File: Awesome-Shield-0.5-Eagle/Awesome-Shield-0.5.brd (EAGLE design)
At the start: 100 x 80 mm, 24 parts, among them J1 ARDUINO_R3_SHIELDUNO_R3_SHIEL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, SW1 SPST_TACT-EVQQ2

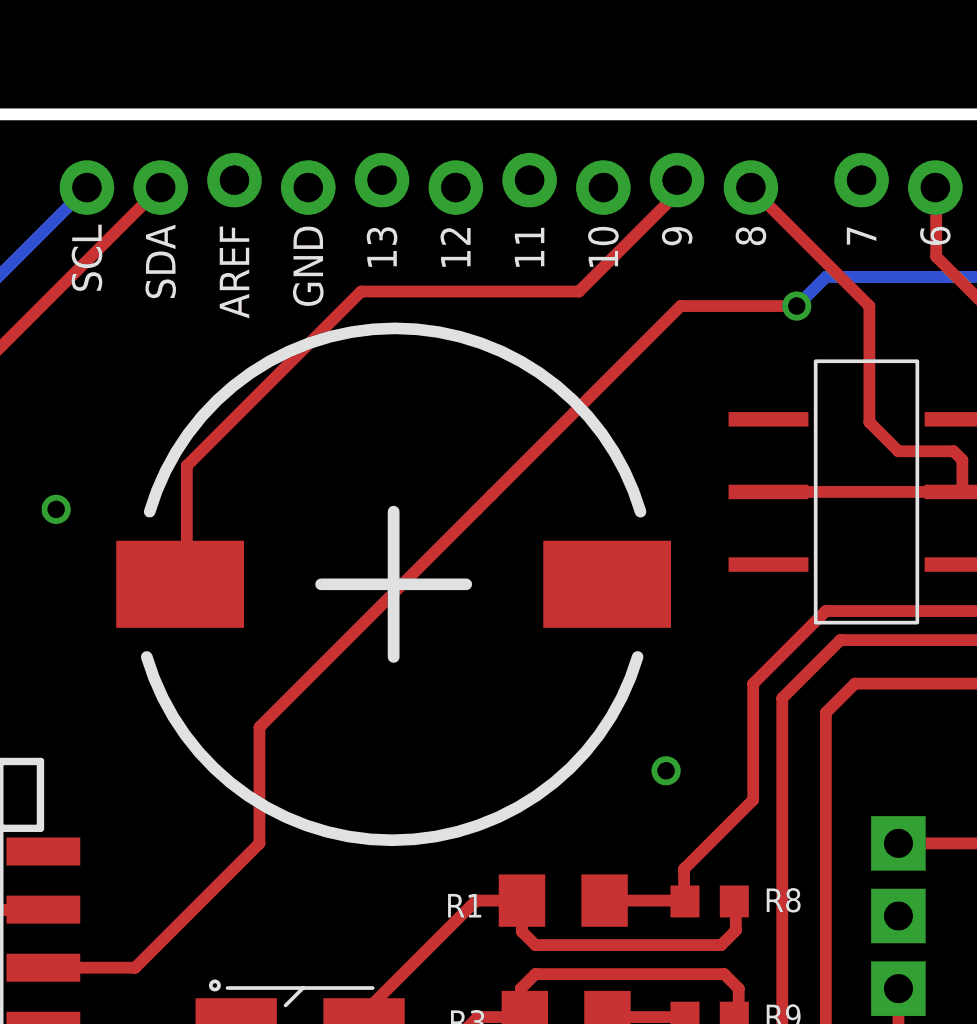
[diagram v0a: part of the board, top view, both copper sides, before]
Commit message: nudged traces
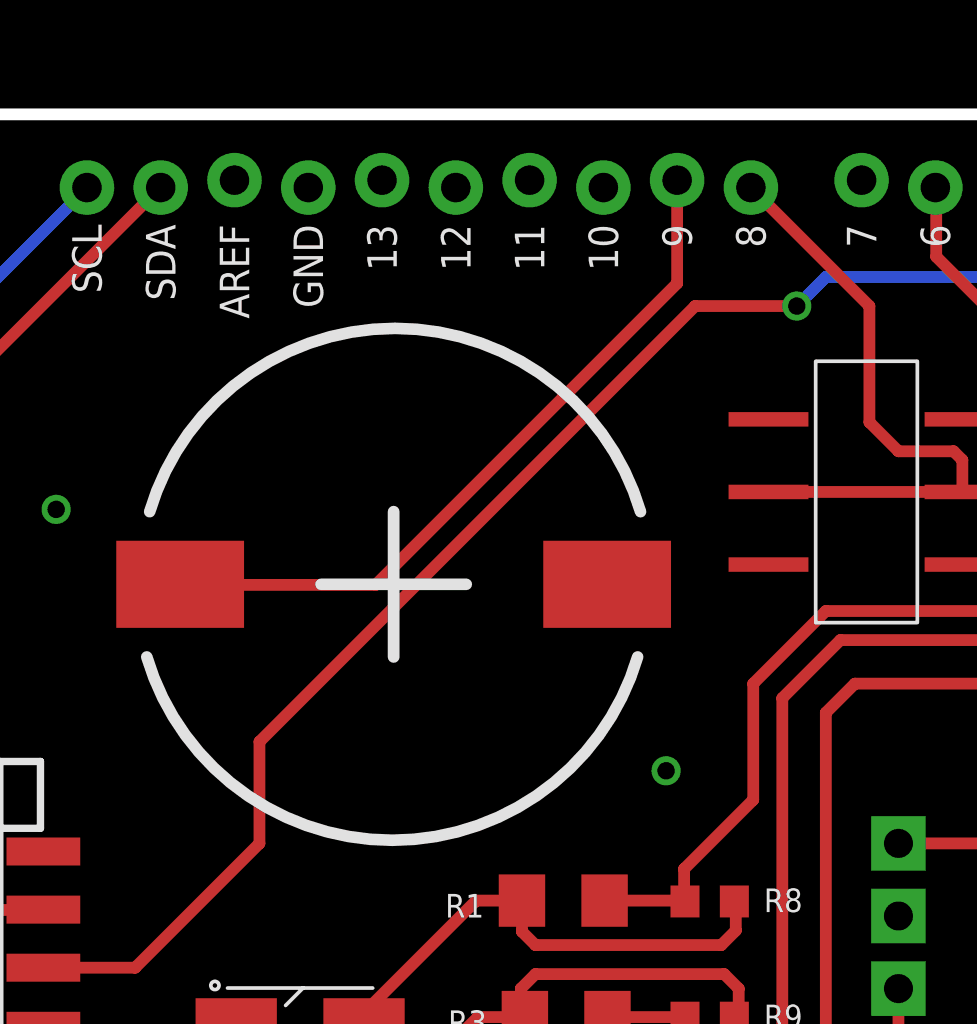
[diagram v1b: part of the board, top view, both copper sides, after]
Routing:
- net D9: track 26.9 -> 25.0 mm
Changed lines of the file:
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@@
 <via x="66.5" y="36.5" extent="1-16" drill="0.6"/>
 <via x="29.5" y="67" extent="1-16" drill="0.6"/>
+<wire x1="79.78" y1="62.58" x2="87.5" y2="73" width="0" layer="19" extent="1-1"/>
 </signal>
 <signal name="A2">
@@
 <contactref element="J1" pad="D9"/>
 <contactref element="SG1" pad="-"/>
-<wire x1="55.88" y1="68.834" x2="55.88" y2="68.38" width="0.4064" layer="1"/>
-<wire x1="55.88" y1="68.38" x2="52.5" y2="65" width="0.4064" layer="1"/>
-<wire x1="52.5" y1="65" x2="45" y2="65" width="0.4064" layer="1"/>
-<wire x1="45" y1="65" x2="39" y2="59" width="0.4064" layer="1"/>
-<wire x1="39" y1="59" x2="39" y2="54.15" width="0.4064" layer="1"/>
-<wire x1="39" y1="54.15" x2="38.77" y2="54.92" width="0.4064" layer="1"/>
+<wire x1="55.88" y1="68.834" x2="55.88" y2="65.28" width="0.4064" layer="1"/>
+<wire x1="45.5" y1="54.9" x2="38.79" y2="54.9" width="0.4064" layer="1"/>
+<wire x1="38.79" y1="54.9" x2="38.77" y2="54.92" width="0.4064" layer="1"/>
+<wire x1="55.88" y1="65.28" x2="45.5" y2="54.9" width="0.4064" layer="1"/>
 </signal>
 <signal name="D4">
@@
 <wire x1="69.8" y1="66" x2="69.8" y2="68.53" width="0.4064" layer="16"/>
 <wire x1="69.8" y1="68.53" x2="69.85" y2="68.58" width="0.4064" layer="16"/>
-<wire x1="49.5" y1="58" x2="49" y2="57.5" width="0.4064" layer="1"/>
-<wire x1="49" y1="57.5" x2="41.5" y2="50" width="0.4064" layer="1"/>
-<wire x1="41.5" y1="50" x2="41.5" y2="46" width="0.4064" layer="1"/>
+<wire x1="41.5" y1="49.5" x2="41.5" y2="46" width="0.4064" layer="1"/>
 <wire x1="41.5" y1="46" x2="37.22" y2="41.72" width="0.4064" layer="1"/>
-<wire x1="60" y1="64.5" x2="56" y2="64.5" width="0.4064" layer="1"/>
-<wire x1="56" y1="64.5" x2="49.5" y2="58" width="0.4064" layer="1"/>
+<wire x1="60" y1="64.5" x2="56.5" y2="64.5" width="0.4064" layer="1"/>
+<wire x1="56.5" y1="64.5" x2="41.5" y2="49.5" width="0.4064" layer="1"/>
 </signal>
 <signal name="N$2">
